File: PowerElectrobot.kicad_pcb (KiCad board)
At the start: 2 copper layers, 58 parts, among them J10 Conn_XT30F, J11 Conn_XT30F, J12 Conn_XT30F, J13 Conn_XT30F, J14 Conn_XT30F, J15 Conn_XT30F, J16 Conn_XT30F, J17 Conn_XT30F, J18 Conn_XT30F, J19 Conn_XT30F, J2 Conn_XT60M, J3 Conn_XT30F, J4 Conn_XT30F, J5 Conn_XT30F, J6 Conn_XT30F, J7 Conn_XT30F, J8 Conn_01x04, J9 Conn_01x04, Q1 BTS117, Q2 BTS117, Q3 BTS117, Q4 BTS117, Q5 BTS117, Q6 BTS117, Q7 BTS117, Q8 BTS117, U1 DSPIC33FJ128MC802-xSP, U2 TSR_2-2450, U3 MCP1804x-3302xDB, U4 ACS712xLCTR-05B, U5 ACS712xLCTR-05B, U6 ACS712xLCTR-20A

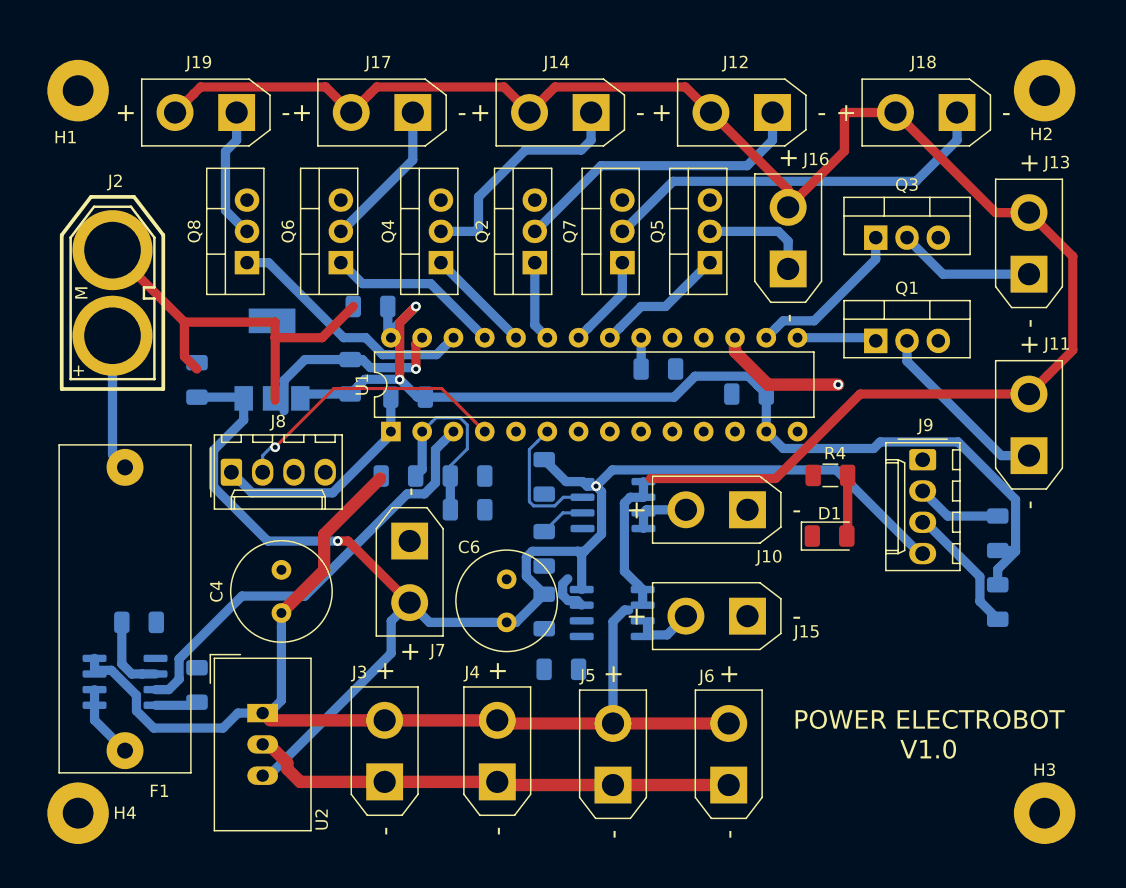
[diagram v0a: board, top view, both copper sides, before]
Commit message: Version initiale du placement de composants
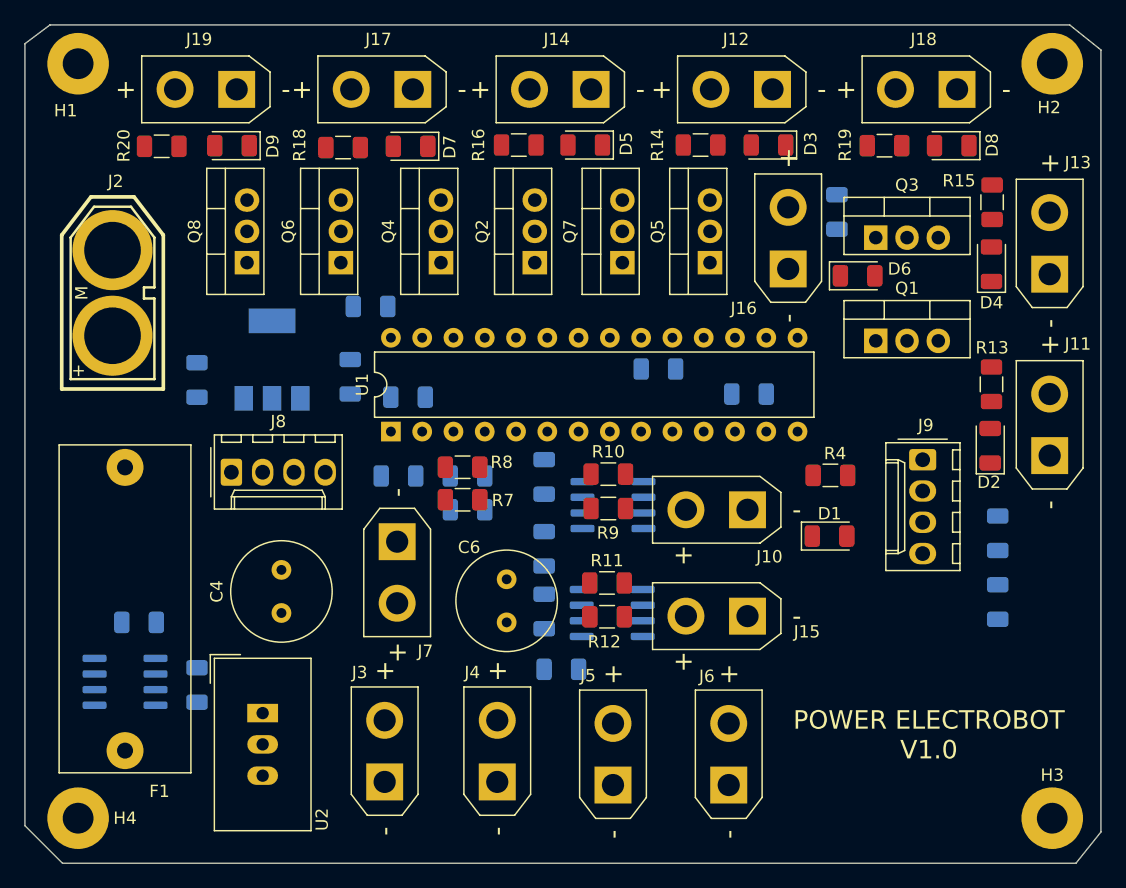
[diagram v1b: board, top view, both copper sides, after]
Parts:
- added D2: LED, LED_SMD:LED_1206_3216Metric, F.Cu at (147.0, 90.0)
- added D3: LED, LED_SMD:LED_1206_3216Metric, F.Cu at (129.0, 65.6)
- added D4: LED, LED_SMD:LED_1206_3216Metric, F.Cu at (147.1, 75.3)
- added D5: LED, LED_SMD:LED_1206_3216Metric, F.Cu at (114.1, 65.6)
- added D6: LED, LED_SMD:LED_1206_3216Metric, F.Cu at (136.2, 76.3)
- added D7: LED, LED_SMD:LED_1206_3216Metric, F.Cu at (99.9, 65.7)
- added D8: LED, LED_SMD:LED_1206_3216Metric, F.Cu at (143.8, 65.7)
- added D9: LED, LED_SMD:LED_1206_3216Metric, F.Cu at (85.4, 65.7)
- added R10: 91k, Resistor_SMD:R_1206_3216Metric, F.Cu at (116.0, 92.4)
- added R11: 47k, Resistor_SMD:R_1206_3216Metric, F.Cu at (115.8, 101.2)
- added R12: 91k, Resistor_SMD:R_1206_3216Metric, F.Cu at (115.9, 103.9)
- added R13: R, Resistor_SMD:R_1206_3216Metric, F.Cu at (147.1, 85.1)
- added R14: R, Resistor_SMD:R_1206_3216Metric, F.Cu at (123.4, 65.6)
- added R15: R, Resistor_SMD:R_1206_3216Metric, F.Cu at (147.1, 70.3)
- added R16: R, Resistor_SMD:R_1206_3216Metric, F.Cu at (108.7, 65.6)
- added R17: R, Resistor_SMD:R_1206_3216Metric, B.Cu at (134.5, 71.1)
- added R18: R, Resistor_SMD:R_1206_3216Metric, F.Cu at (94.4, 65.8)
- added R19: R, Resistor_SMD:R_1206_3216Metric, F.Cu at (138.4, 65.7)
- added R20: R, Resistor_SMD:R_1206_3216Metric, F.Cu at (79.7, 65.7)
- added R7: 47k, Resistor_SMD:R_1206_3216Metric, F.Cu at (104.1, 94.4)
- added R8: 91k, Resistor_SMD:R_1206_3216Metric, F.Cu at (104.1, 91.8)
- added R9: 47k, Resistor_SMD:R_1206_3216Metric, F.Cu at (116.0, 95.1)
- C8: value 1u -> 47u
- R4: value 4.7k -> 470
- moved H2 2.27 mm to (152.0, 59.0)
- moved H1 2.18 mm to (72.9, 59.0)
- moved J12 1.88 mm to (129.3, 61.1)
- moved J14 1.88 mm to (114.6, 61.1)
- moved J17 1.88 mm to (100.1, 61.1)
- moved J18 1.88 mm to (144.3, 61.1)
- moved J19 1.88 mm to (85.8, 61.1)
- moved J11 1.68 mm to (151.8, 90.9)
- moved J13 1.68 mm to (151.8, 76.1)
- moved J7 1.02 mm to (98.8, 97.8)
- moved H3 0.74 mm to (152.0, 120.3)
- moved H4 0.41 mm to (72.9, 120.3)
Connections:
- U4 pad 7: /MEAS_CURR_1 -> Net-(R9-Pad2)
- U5 pad 7: /MEAS_CURR_2 -> Net-(R11-Pad2)
- U6 pad 7: /MEAS_CURR_VBAT -> Net-(R7-Pad2)
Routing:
- net /VBAT: track 239.1 -> 0.00 mm
- net +5V: track 119.9 -> 0.00 mm, vias 2 -> 0
- net GND: track 90.1 -> 0.00 mm, vias 1 -> 0
- net /3.3V_dsPIC: track 87.9 -> 0.00 mm, vias 3 -> 0
- net /MEAS_CURR_VBAT: track 35.4 -> 0.00 mm
- net Net-(D8-Pad1): track 32.5 -> 0.00 mm
- net Net-(D3-Pad1): track 23.9 -> 0.00 mm
- net /dsPIC_PGED1: track 23.1 -> 0.00 mm, vias 1 -> 0
- net /dsPIC_Stor8: track 20.4 -> 0.00 mm
- net Net-(D5-Pad1): track 19.0 -> 0.00 mm
- net /dsPIC_MCLR: track 18.6 -> 0.00 mm
- net /I2C_SCL1: track 17.6 -> 0.00 mm, vias 1 -> 0
- net /VBAT_f: track 15.7 -> 0.00 mm
- net Net-(D2-Pad1): track 14.7 -> 0.00 mm
- net /dsPIC_Stor7: track 14.2 -> 0.00 mm
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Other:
- board outline added: 87.4 x 68.1 mm
